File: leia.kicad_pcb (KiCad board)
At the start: 4 copper layers, 43 x 66 mm, 80 parts, among them P1 GND, P1000 ISO7816_NO, P3000 USB_FS_OTG, P513 TP1, P514 TP2, P515 TP3, P523 UART4, P542 TP4, P543 TP5, P545 TP7, P546 TP8, P547 TP9, P548 TP10, P572 DEBUG/PROG, P592 UART1, P595 I2C1_SCL, P596 I2C1_SDA, P6000 USB_FS_OTG, P828 XI, SW503 DFU, SW514 RESET, U1 LD1117S33TR, U300 USBLC6-2, U500 STM32F439VIT6, U600 USBLC6-2, U800 USB3300, Y2 ASEMB-24.000MHZ-LY-T

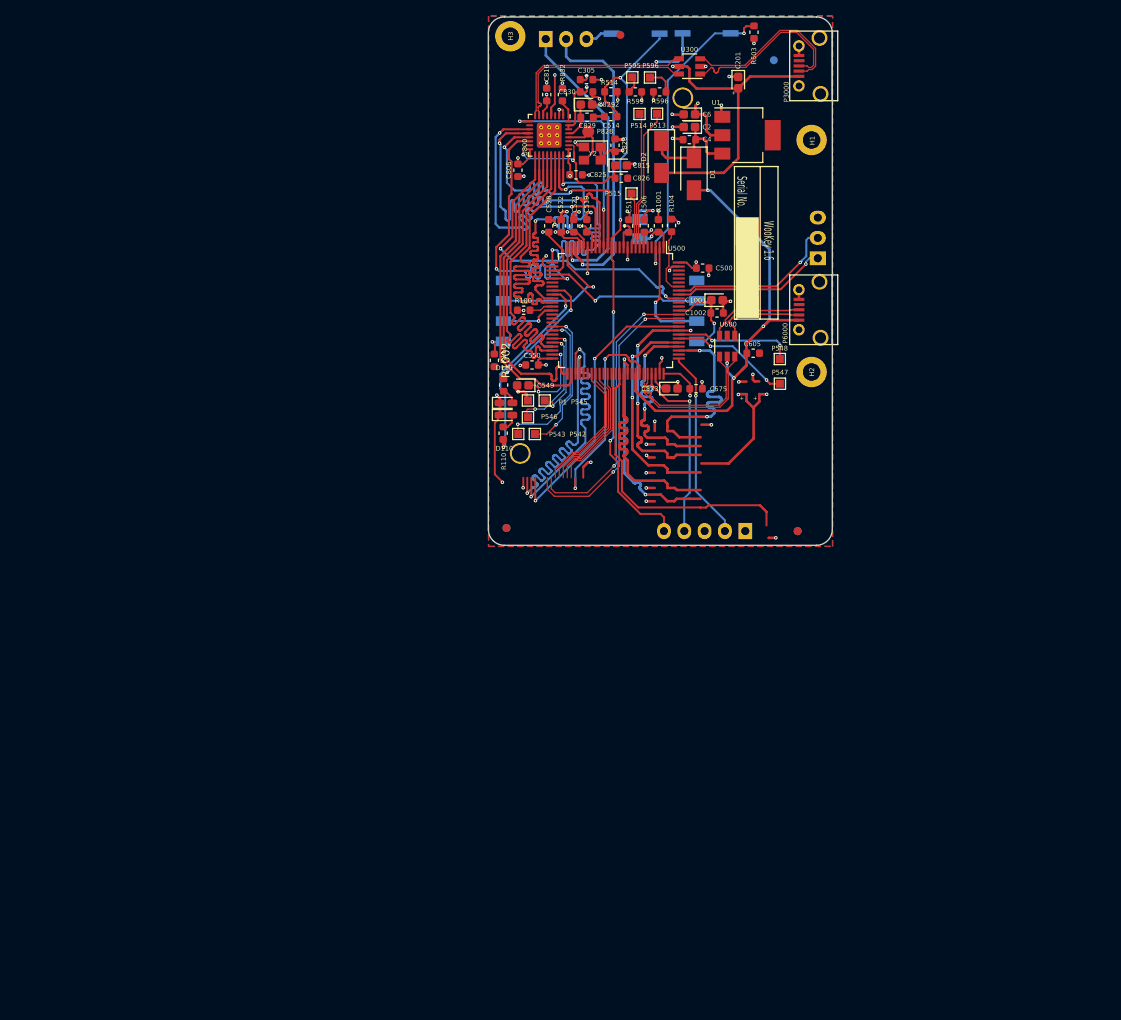
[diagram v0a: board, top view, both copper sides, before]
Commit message: [enhancement] add new file for chipwhisperer interface:iface_ufo.sch
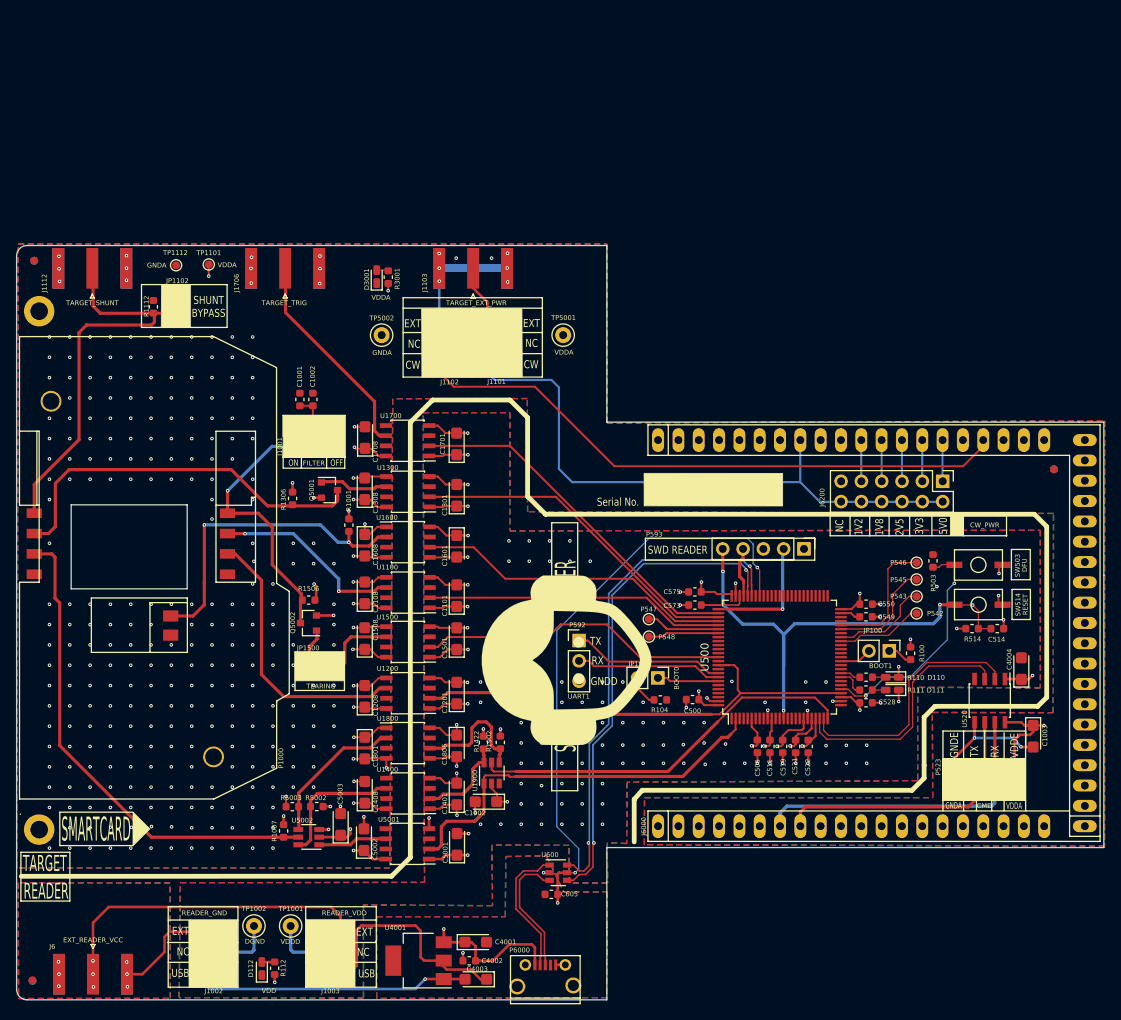
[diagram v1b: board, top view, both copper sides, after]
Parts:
- removed C2, C6: 10uF, Capacitor_Tantalum_SMD:CP_EIA-1608-08_AVX-J
- removed C201, C815, C8292: 4.7uF, Capacitor_Tantalum_SMD:CP_EIA-1608-08_AVX-J
- removed C305, C4, C806, C816, C825, C826, C829, C830: 100nF, Capacitor_SMD:C_0603_1608Metric
- removed C828: 0.01uF, Capacitor_SMD:C_0603_1608Metric
- removed D1, D2: STPS1L30A, Diode_SMD:D_SMA
- removed FID1, FID2, FID3: FIDUCIAL, Fiducials:Fiducial_1mm_Dia_2.54mm_Outer_CopperTop
- removed FID4, FID5, FID6: FIDUCIAL, Fiducials:Fiducial_1mm_Dia_2.54mm_Outer_CopperBottom
- removed H1: H1, Mounting_Holes:MountingHole_2.2mm_M2_ISO14580_Pad
- removed H2: H2, Mounting_Holes:MountingHole_2.2mm_M2_ISO14580_Pad
- removed H3: H3, Mounting_Holes:MountingHole_2.2mm_M2_ISO14580_Pad
- removed P1: GND, TestPoint:TestPoint_Pad_1.0x1.0mm
- removed P3000: USB_FS_OTG, leia:USB_Micro-B-MOLEX_105017-0001
- removed P513: TP1, TestPoint:TestPoint_Pad_1.0x1.0mm
- removed P514: TP2, TestPoint:TestPoint_Pad_1.0x1.0mm
- removed P515: TP3, TestPoint:TestPoint_Pad_1.0x1.0mm
- removed P572: DEBUG/PROG, Pin_Headers:Pin_Header_Straight_1x05
- removed P595: I2C1_SCL, TestPoint:TestPoint_Pad_1.0x1.0mm
- removed P596: I2C1_SDA, TestPoint:TestPoint_Pad_1.0x1.0mm
- removed P828: XI, Measurement_Points:Measurement_Point_Round-SMD-Pad_Small
- removed R1002: 10, Resistor_SMD:R_0603_1608Metric
- removed R595, R596: 47K, Resistor_SMD:R_0603_1608Metric
- removed R832: 12K [1%], Resistor_SMD:R_0603_1608Metric
- removed U1: LD1117S33TR, Package_TO_SOT_SMD:SOT-223
- removed U300: USBLC6-2, Package_TO_SOT_SMD:TSOT-23-6
- removed U800: USB3300, Package_DFN_QFN:QFN-32-1EP_5x5mm_P0.5mm_EP3.1x3.1mm_ThermalVias
- removed Y2: ASEMB-24.000MHZ-LY-T, Oscillator:Oscillator_SMD_Abracon_ASE-4Pin_3.2x2.5mm
- added C1003: 0.1uF 35V Tant, Capacitor_Tantalum_SMD:CP_EIA-3216-18_Kemet-A, F.Cu at (154.1, 129.7)
- added C1101: 0.1uF 35V Tant, Capacitor_Tantalum_SMD:CP_EIA-3216-18_Kemet-A, F.Cu at (82.0, 112.1)
- added C1108: 0.1uF 35V Tant, Capacitor_Tantalum_SMD:CP_EIA-3216-18_Kemet-A, F.Cu at (70.5, 111.8)
- added C1201: 0.1uF 35V Tant, Capacitor_Tantalum_SMD:CP_EIA-3216-18_Kemet-A, F.Cu at (82.0, 124.3)
- added C1208: 0.1uF 35V Tant, Capacitor_Tantalum_SMD:CP_EIA-3216-18_Kemet-A, F.Cu at (70.5, 124.7)
- added C1301: 0.1uF 35V Tant, Capacitor_Tantalum_SMD:CP_EIA-3216-18_Kemet-A, F.Cu at (82.0, 99.6)
- added C1308: 0.1uF 35V Tant, Capacitor_Tantalum_SMD:CP_EIA-3216-18_Kemet-A, F.Cu at (70.5, 98.8)
- added C1401: 0.1uF 35V Tant, Capacitor_Tantalum_SMD:CP_EIA-3216-18_Kemet-A, F.Cu at (82.0, 136.9)
- added C1408: 0.1uF 35V Tant, Capacitor_Tantalum_SMD:CP_EIA-3216-18_Kemet-A, F.Cu at (70.5, 136.7)
- added C1501: 0.1uF 35V Tant, Capacitor_Tantalum_SMD:CP_EIA-3216-18_Kemet-A, F.Cu at (82.0, 117.5)
- added C1508: 0.1uF 35V Tant, Capacitor_Tantalum_SMD:CP_EIA-3216-18_Kemet-A, F.Cu at (70.5, 117.5)
- added C1601: 0.1uF 35V Tant, Capacitor_Tantalum_SMD:CP_EIA-3216-18_Kemet-A, F.Cu at (82.0, 106.0)
- added C1608: 0.1uF 35V Tant, Capacitor_Tantalum_SMD:CP_EIA-3216-18_Kemet-A, F.Cu at (70.5, 105.8)
- added C1701: 0.1uF 35V Tant, Capacitor_Tantalum_SMD:CP_EIA-3216-18_Kemet-A, F.Cu at (82.0, 93.2)
- added C1708: 0.1uF 35V Tant, Capacitor_Tantalum_SMD:CP_EIA-3216-18_Kemet-A, F.Cu at (70.6, 92.4)
- added C1801: 0.1uF 35V Tant, Capacitor_Tantalum_SMD:CP_EIA-3216-18_Kemet-A, F.Cu at (70.5, 131.2)
- added C1806: 0.1uF 35V Tant, Capacitor_Tantalum_SMD:CP_EIA-3216-18_Kemet-A, F.Cu at (82.0, 130.9)
- added C1902: 0.1uF 35V Tant, Capacitor_Tantalum_SMD:CP_EIA-3216-18_Kemet-A, F.Cu at (85.7, 137.9)
- added C4001: 10uF, Capacitor_Tantalum_SMD:CP_EIA-3216-18_Kemet-A, F.Cu at (84.4, 155.4)
- added C4002: 100nF, Capacitor_SMD:C_0603_1608Metric, F.Cu at (83.6, 157.8)
- added C4003: 10uF, Capacitor_Tantalum_SMD:CP_EIA-3216-18_Kemet-A, F.Cu at (84.4, 160.1)
- added C4004: 0.1uF 35V Tant, Capacitor_Tantalum_SMD:CP_EIA-3216-18_Kemet-A, F.Cu at (152.6, 121.3)
- added C5001: 0.1uF 35V Tant, Capacitor_Tantalum_SMD:CP_EIA-3216-18_Kemet-A, F.Cu at (82.1, 143.2)
- added C5002: 0.1uF 35V Tant, Capacitor_Tantalum_SMD:CP_EIA-3216-18_Kemet-A, F.Cu at (70.4, 142.6)
- added C5003: 0.1uF 35V Tant, Capacitor_Tantalum_SMD:CP_EIA-3216-18_Kemet-A, F.Cu at (67.5, 140.7)
- added D112: VDD, LED_SMD:LED_0603_1608Metric_Castellated, F.Cu at (57.7, 158.8)
- added D3001: VDDA, LED_SMD:LED_0603_1608Metric_Castellated, F.Cu at (72.0, 72.3)
- added FID1001: FIDUCIAL-RESCUE-rescue, Fiducial:Fiducial_1mm_Mask2mm, B.Cu at (29.0, 160.3)
- added FID1002: FIDUCIAL-RESCUE-rescue, Fiducial:Fiducial_1mm_Mask2mm, F.Cu at (29.2, 70.3)
- added FID1003: FIDUCIAL-RESCUE-rescue, Fiducial:Fiducial_1mm_Mask2mm, B.Cu at (29.2, 70.3)
- added FID1004: FIDUCIAL-RESCUE-rescue, Fiducial:Fiducial_1mm_Mask2mm, F.Cu at (156.7, 96.3)
- added FID1005: FIDUCIAL-RESCUE-rescue, Fiducial:Fiducial_1mm_Mask2mm, B.Cu at (156.7, 96.3)
- added FID1006: FIDUCIAL-RESCUE-rescue, Fiducial:Fiducial_1mm_Mask2mm, F.Cu at (29.0, 160.2)
- added G***: LOGO, leia:Leia-medium, F.Cu at (95.8, 120.2)
- added HOLE1: HOLE, MountingHole:MountingHole_2.2mm_M2_ISO14580_Pad, F.Cu at (29.8, 141.4)
- added HOLE2: HOLE, MountingHole:MountingHole_2.2mm_M2_ISO14580_Pad, F.Cu at (29.8, 76.6)
- added J1001: FILTER, Connector_PinHeader_2.54mm:PinHeader_2x03_P2.54mm_Vertical, F.Cu at (61.7, 93.5)
- added J1002: READER_GND, Connector_PinHeader_2.54mm:PinHeader_2x03_P2.54mm_Vertical, F.Cu at (52.9, 159.2)
- added J1003: READER_VDD, Connector_PinHeader_2.54mm:PinHeader_2x03_P2.54mm_Vertical, F.Cu at (67.5, 159.2)
- added J1101: TARGET_PWR, Connector_PinHeader_2.54mm:PinHeader_2x03_P2.54mm_Vertical, F.Cu at (88.4, 83.1)
- added J1102: TARGET_GND, Connector_PinHeader_2.54mm:PinHeader_2x03_P2.54mm_Vertical, F.Cu at (82.0, 83.1)
- added J1103: TARGET_EXT_PWR, Connector_Coaxial:SMA_Amphenol_132289_EdgeMount, F.Cu at (84.1, 71.2)
- added J1112: TARGET_SHUNT, Connector_Coaxial:SMA_Amphenol_132289_EdgeMount, F.Cu at (36.5, 71.2)
- added J1706: TARGET_TRIG, Connector_Coaxial:SMA_Amphenol_132289_EdgeMount, F.Cu at (60.6, 71.2)
- added J6: EXT_READER_VCC, Connector_Coaxial:SMA_Amphenol_132289_EdgeMount, F.Cu at (36.6, 159.5)
- added J6000: CW308_TARGETCON, leia:CW308T_CONNBOARD, F.Cu at (107.2, 141.0)
- added J6200: CW_PWR, Connector_PinHeader_2.54mm:PinHeader_2x06_P2.54mm_Vertical, F.Cu at (142.8, 97.8)
- added JP100: BOOT1, Connector_PinHeader_2.54mm:PinHeader_1x02_P2.54mm_Vertical, F.Cu at (136.1, 119.0)
- added JP101: BOOT0, Connector_PinHeader_2.54mm:PinHeader_1x02_P2.54mm_Vertical, F.Cu at (107.2, 122.4)
- added JP1102: SHUNT Bypass, Connector_PinHeader_2.54mm:PinHeader_1x02_P2.54mm_Vertical, F.Cu at (46.9, 77.2)
- added JP1500: TEARING, Connector_PinHeader_2.54mm:PinHeader_1x02_P2.54mm_Vertical, F.Cu at (66.2, 121.0)
- added P593: SWD, Connector_PinHeader_2.54mm:PinHeader_1x05_P2.54mm_Vertical, F.Cu at (125.4, 106.3)
- added Q5001: BSS84, Package_TO_SOT_SMD:SOT-23, F.Cu at (66.1, 98.9)
- added Q5002: BSS84, Package_TO_SOT_SMD:SOT-23, F.Cu at (63.5, 115.6)
- added R1007: 22k, Resistor_SMD:R_0603_1608Metric, F.Cu at (60.4, 141.6)
- added R1112: 0.1 1%, Resistor_SMD:R_0603_1608Metric, F.Cu at (44.1, 76.0)
- added R112: 470, Resistor_SMD:R_0603_1608Metric, F.Cu at (59.3, 158.7)
- added R1306: 10k, Resistor_SMD:R_0603_1608Metric, F.Cu at (61.5, 100.0)
- added R1422: 22k, Resistor_SMD:R_0603_1608Metric, F.Cu at (85.4, 130.5)
- added R1506: 10k, Resistor_SMD:R_0603_1608Metric, F.Cu at (63.5, 112.7)
- added R1902: 22k, Resistor_SMD:R_0603_1608Metric, F.Cu at (87.5, 130.5)
- added R3001: 470, Resistor_SMD:R_0603_1608Metric, F.Cu at (73.5, 72.3)
- added R5002: DNP, Resistor_SMD:R_0603_1608Metric, F.Cu at (64.5, 138.5)
- added R5003: DNP, Resistor_SMD:R_0603_1608Metric, F.Cu at (61.5, 138.5)
- added TP1001: VDDD, TestPoint_Keystone_5000-5004_Miniature, F.Cu at (61.3, 153.4)
- added TP1002: DGND, TestPoint_Keystone_5000-5004_Miniature, F.Cu at (56.7, 153.4)
- added TP1101: VDDA, TestPoint:TestPoint_Pad_D1.0mm, F.Cu at (51.0, 70.7)
- added TP1112: GNDA, TestPoint:TestPoint_Pad_D1.0mm, F.Cu at (46.9, 70.8)
- added TP5001: VDDA, TestPoint_Keystone_5000-5004_Miniature, F.Cu at (95.3, 79.6)
- added TP5002: GNDA, TestPoint_Keystone_5000-5004_Miniature, F.Cu at (72.6, 79.6)
- added U1100: FOD8001, Package_SO:SOIC-8_3.9x4.9mm_P1.27mm, F.Cu at (75.9, 111.8)
- added U1200: FOD8001, Package_SO:SOIC-8_3.9x4.9mm_P1.27mm, F.Cu at (75.9, 124.3)
- added U1300: FOD8001, Package_SO:SOIC-8_3.9x4.9mm_P1.27mm, F.Cu at (75.9, 99.2)
- added U1400: FOD8001, Package_SO:SOIC-8_3.9x4.9mm_P1.27mm, F.Cu at (75.9, 136.9)
- added U1500: FOD8001, Package_SO:SOIC-8_3.9x4.9mm_P1.27mm, F.Cu at (75.9, 117.9)
- added U1600: FOD8001, Package_SO:SOIC-8_3.9x4.9mm_P1.27mm, F.Cu at (75.9, 105.5)
- added U1700: FOD8001, Package_SO:SOIC-8_3.9x4.9mm_P1.27mm, F.Cu at (75.9, 92.8)
- added U1800: FOD8001, Package_SO:SOIC-8_3.9x4.9mm_P1.27mm, F.Cu at (75.9, 130.6)
- added U1900: ADG719-EP, Package_TO_SOT_SMD:TSOT-23-6, F.Cu at (86.4, 134.3)
- added U4001: LD1117S33TR, Package_TO_SOT_SMD:SOT-223, F.Cu at (77.3, 157.8)
- added U5001: FOD8001, Package_SO:SOIC-8_3.9x4.9mm_P1.27mm, F.Cu at (75.9, 143.2)
- added U5002: ADG719-EP, Package_TO_SOT_SMD:TSOT-23-6, F.Cu at (63.5, 142.3)
- added U520: FOD8012A, Package_SO:SOIC-8_3.9x4.9mm_P1.27mm, F.Cu at (148.7, 125.3)
- C1001, C549, C573: footprint Capacitor_Tantalum_SMD:CP_EIA-1608-08_AVX-J -> Capacitor_SMD:C_0603_1608Metric
- P1000, SW503, SW514: moved to F.Cu
- P523: value UART4 -> CMD; footprint Pin_Headers:Pin_Header_Straight_1x03 -> Connector_PinHeader_2.54mm:PinHeader_2x04_P2.54mm_Vertical; moved to F.Cu
- P542, P543, P545, P546, P547, P548: footprint TestPoint:TestPoint_Pad_1.0x1.0mm -> TestPoint:TestPoint_Pad_D1.0mm
- P592: footprint Pin_Headers:Pin_Header_Straight_1x03 -> Connector_PinHeader_2.54mm:PinHeader_1x03_P2.54mm_Vertical; moved to F.Cu
- P6000: value USB_FS_OTG -> USB_FS
- R1001: value 10K -> 20k
- U500: footprint Housings_QFP:LQFP-100_14x14mm_Pitch0.5mm -> Package_QFP:TQFP-100_14x14mm_P0.5mm
- U600: footprint Package_TO_SOT_SMD:TSOT-23-6 -> Package_TO_SOT_SMD:SOT-23-6
- moved P523 108.5 mm to (151.8, 133.8)
- moved P1000 101.2 mm to (51.6, 132.3), turned to 270 degrees
- moved P6000 91.3 mm to (93.1, 161.0), turned to 0 degrees
- moved SW514 83.3 mm to (147.2, 113.3)
- moved R514 80.9 mm to (146.4, 116.3), turned to 0 degrees
- moved C514 80.2 mm to (149.6, 116.3), turned to 0 degrees
- moved SW503 74.6 mm to (147.2, 108.3)
- moved C605 72.2 mm to (93.9, 149.5), turned to 180 degrees
- moved C522 72.0 mm to (126.0, 131.0), turned to 270 degrees
- moved C528 71.6 mm to (133.2, 125.5), turned to 0 degrees
- moved C521 70.7 mm to (124.4, 131.0), turned to 270 degrees
- moved R503 69.8 mm to (141.6, 107.8), turned to 90 degrees
- moved C519 69.5 mm to (122.8, 131.0), turned to 270 degrees
- moved U600 69.1 mm to (94.7, 146.8), turned to 0 degrees
- moved C511 67.4 mm to (121.2, 131.0), turned to 270 degrees
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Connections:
- net LED0 renamed /cpu/LED0_PC4
- net LED1 renamed /cpu/LED1_PC5
- C1001 pad 1: /cpu/CARD_POWER -> Net-(C1001-Pad1)
- C1001 pad 2: GND -> GNDA
- C1002 pad 1: /cpu/CARD_POWER -> Net-(C1001-Pad1)
- C1002 pad 2: GND -> GNDA
- C500 pad 1: +3V3 -> VDD
- C500 pad 2: GND -> GNDD
- C506 pad 1: +3V3 -> VDD
- C506 pad 2: GND -> GNDD
- C511 pad 1: +3V3 -> VDD
- C511 pad 2: GND -> GNDD
- C514 pad 2: GND -> GNDD
- C519 pad 1: +3V3 -> VDD
- C519 pad 2: GND -> GNDD
- C521 pad 1: +3V3 -> VDD
- C521 pad 2: GND -> GNDD
- C522 pad 1: +3V3 -> VDD
- C522 pad 2: GND -> GNDD
- C528 pad 1: +3V3 -> VDD
- C528 pad 2: GND -> GNDD
- C549 pad 2: GND -> GNDD
- C550 pad 1: +3V3 -> VDD
- C550 pad 2: GND -> GNDD
- C573 pad 2: GND -> GNDD
- C575 pad 1: +3V3 -> VDD
- C575 pad 2: GND -> GNDD
- C605 pad 2: GND -> GNDPWR
- D110 pad 1: GND -> GNDD
- D111 pad 1: GND -> GNDD
- P1000 pad C1: /cpu/CARD_POWER -> /dfu smartcard/CRD_PWR
- P1000 pad C2: /cpu/CARD_RESET -> /dfu smartcard/CRD_RST
- P1000 pad C3: /cpu/CARD_CLK -> /dfu smartcard/CRD_CLK
- P1000 pad C5: Net-(P1000-PadC5) -> /GNDCARD
- P1000 pad C6: /cpu/CARD_VPP -> /dfu smartcard/CRD_VPP
- P1000 pad C7: /cpu/CARD_IO -> /dfu smartcard/CRD_IO
- P1000 pad SW1: /cpu/CARD_CT -> /dfu smartcard/CRD_CT
- P1000 pad SW2: GND -> GNDA
- P523 pad 1: /cpu/UART4_RX_PA1 -> /VDD_CONSOLE
- P523 pad 2: /cpu/UART4_TX_PA0 -> VDDA
- P523 pad 3: GND -> /RX_CONSOLE
- P592 pad 3: GND -> GNDD
- P6000 pad 5: GND -> GNDPWR
- P6000 pad 6: GND -> GNDPWR
- R100 pad 1: +3V3 -> VDD
- R100 pad 2: /cpu/BOOT1 -> Net-(JP100-Pad1)
- R1001 pad 1: +3V3 -> VDDA
- R1001 pad 2: /cpu/CARD_CT -> /dfu smartcard/CRD_CT
- R104 pad 1: /cpu/BOOT0 -> Net-(JP101-Pad2)
- R104 pad 2: GND -> GNDD
- R503 pad 2: GND -> GNDD
- R514 pad 1: +3V3 -> VDD
- SW503 pad 1: +3V3 -> VDD
- SW514 pad 2: GND -> GNDD
- U500 pad 1: /cpu/CARD_CT -> (no net)
- U500 pad 10: GND -> GNDD
- U500 pad 100: +3V3 -> VDD
- U500 pad 11: +3V3 -> VDD
- U500 pad 15: /cpu/USB_HS_ULPI_STP -> (no net)
- U500 pad 16: /cpu/USB_HS_HARD_RESET -> (no net)
- U500 pad 17: /cpu/USB_HS_ULPI_DIR -> (no net)
- U500 pad 18: /cpu/USB_HS_ULPI_NXT -> (no net)
- U500 pad 19: +3V3 -> VDD
- U500 pad 2: /cpu/CARD_RESET -> /cpu/CARD_~R~W
- U500 pad 20: GND -> GNDD
- U500 pad 21: +3V3 -> VDD
- U500 pad 22: +3V3 -> VDD
- U500 pad 23: /cpu/UART4_TX_PA0 -> /TX_CMD
- U500 pad 24: /cpu/UART4_RX_PA1 -> /RX_CMD
- U500 pad 26: /cpu/USB_HS_ULPI_D0 -> (no net)
- U500 pad 27: GND -> GNDD
- U500 pad 28: +3V3 -> VDD
- U500 pad 3: /cpu/DFU -> (no net)
- U500 pad 30: /cpu/USB_HS_ULPI_CLK -> /cpu/DFU
- U500 pad 35: /cpu/USB_HS_ULPI_D1 -> (no net)
- U500 pad 36: /cpu/USB_HS_ULPI_D2 -> (no net)
- U500 pad 38: /cpu/CARD_VPP -> (no net)
- U500 pad 47: /cpu/USB_HS_ULPI_D3 -> (no net)
- U500 pad 48: /cpu/USB_HS_ULPI_D4 -> (no net)
- U500 pad 50: +3V3 -> VDD
- U500 pad 51: /cpu/USB_HS_ULPI_D5 -> (no net)
- U500 pad 52: /cpu/USB_HS_ULPI_D6 -> (no net)
- U500 pad 6: +3V3 -> VDD
- U500 pad 7: /cpu/TP1 -> (no net)
- U500 pad 72: /cpu/TMS/SWIO -> /cpu/TMS
- U500 pad 74: GND -> GNDD
- U500 pad 75: +3V3 -> VDD
- U500 pad 76: /cpu/TCK/SWCLK -> /cpu/TCK
- U500 pad 77: (no net) -> /cpu/TRIGGER
- U500 pad 78: (no net) -> /cpu/CARD_VPP
- U500 pad 79: (no net) -> /cpu/CARD_CT
- U500 pad 8: /cpu/TP2 -> (no net)
- U500 pad 80: (no net) -> /cpu/CARD_RESET
- U500 pad 88: /cpu/CARD_POWER -> /cpu/CARD_PWR_EN
- U500 pad 9: /cpu/TP3 -> (no net)
- U500 pad 90: (no net) -> /cpu/CARD_CLK
- U500 pad 91: /cpu/USB_HS_ULPI_D7 -> (no net)
- U500 pad 99: GND -> GNDD
- U600 pad 2: GND -> GNDPWR
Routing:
- net (no net): track 493.1 -> 0.00 mm, vias 23 -> 0
- net VDD: track 0.00 -> 110.0 mm, vias 0 -> 26
- net +3V3: track 108.5 -> 0.00 mm, vias 31 -> 0
- net GNDD: track 0.00 -> 80.4 mm, vias 0 -> 118
- net VCOM: track 0.00 -> 78.1 mm
- net VDDA: track 0.00 -> 61.4 mm, vias 0 -> 18
- net /dfu smartcard/CRD_IO: track 0.00 -> 61.1 mm
- net /cpu/CARD_~R~W: track 0.00 -> 53.7 mm
- net /GNDCARD: track 0.00 -> 51.7 mm
- net /dfu smartcard/CRD_VPP: track 0.00 -> 47.9 mm
- net /cpu/USB_HS_ULPI_D1: track 46.8 -> 0.00 mm, vias 2 -> 0
- net /cpu/USB_HS_VBUS: track 45.8 -> 0.00 mm, vias 3 -> 0
- net /cpu/TRIGGER: track 0.00 -> 44.6 mm
- net /cpu/USB_HS_ULPI_DIR: track 44.3 -> 0.00 mm, vias 2 -> 0
- net /cpu/USB_FS_D-: track 19.9 -> 61.7 mm, vias 0 -> 2
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- added copper zone on B.Cu, net /EXT_READER_GND
- added copper zone on F.Cu, net /EXT_READER_GND
- added copper zone on In1.Cu, net /EXT_READER_GND
- added copper zone on In2.Cu, net /EXT_READER_VCC
- added copper zone on In2.Cu, net /cpu/USB_FS_VBUS
- added copper zone on B.Cu, net GNDA
- added copper zone on F.Cu, net GNDA
- added copper zone on In1.Cu, net GNDA
- added copper zone on B.Cu, net GNDD
- added copper zone on F.Cu, net GNDD
- added copper zone on In1.Cu, net GNDD
- added copper zone on B.Cu, net GNDPWR
- added copper zone on F.Cu, net GNDPWR
- added copper zone on In1.Cu, net GNDPWR
- added copper zone on In2.Cu, net VDD
- added copper zone on In2.Cu, net VDDA
- removed copper zone on In2Power.Cu, net +3V3
- removed copper zone on In2Power.Cu, net /cpu/USB_FS_VBUS
- removed copper zone on In2Power.Cu, net /cpu/USB_HS_VBUS
- removed copper zone on B.Cu, net GND
- removed copper zone on F.Cu, net GND
- removed copper zone on In1GroundPlan.Cu, net GND
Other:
- board size 43 x 66 mm -> 135.9 x 94.3 mm
- net class Default: clearance 0.127 -> 0.2; via_dia 0.44 -> 0.8; via_drill 0.2 -> 0.4
- net class Power: clearance 0.127 -> 0.15; trace_width 0.127 -> 0.25
- rule trace_clearance: 0.127 -> 0.2
- rule via_min_size: 0.44 -> 0.2
- board text added: "1"
- board text added: "10"
- board text added: "11"
- board text added: "12"
- board text added: "13"
- board text added: "14"
- board text added: "15"
- board text added: "16"
- board text added: "17"
- board text added: "18"
- board text added: "19"
- board text added: "1V2"
- board text added: "1V8"
- board text added: "2"
- board text added: "20"
- board text added: "21"
- board text added: "22"
- board text added: "23"
- board text added: "24"
- board text added: "25"
- board text added: "26"
- board text added: "27"
- board text added: "28"
- board text added: "29"
- board text added: "2V5"
- board text added: "3"
- board text added: "30"
- board text added: "31/32"
- board text added: "33/34"
- board text added: "35/36"
- board text added: "37/38"
- board text added: "39/40"
- board text added: "3V3"
- board text added: "4"
- board text added: "5"
- board text added: "5V0"
- board text added: "6"
- board text added: "7"
- board text added: "8"
- board text added: "9"
- board text added: "CW"
- board text added: "EXT"
- board text added: "GNDA"
- board text added: "GNDD"
- board text added: "GNDE"
- board text added: "NC"
- board text added: "OFF"
- board text added: "ON"
- board text added: "READER"
- board text added: "RX"
- board text added: "SHUNT BYPASS"
- board text added: "SMART READER"
- board text added: "SMARTCARD"
- board text added: "SWD READER"
- board text added: "TARGET"
- board text added: "TX"
- board text added: "The board is a 4 Layer Stackup is as follows: ============================================ Solder resist: 20 µm Cu - L1 (TOP): 35 µm PP - 1 : 175 µm (7628LR) e = 4.2 Cu - L2 : 17.5 µm Core - 1 : 1150 µm e = 4.3 Cu - L3 : 17.5 µm PP - 2 : 175 µm (7628LR) e = 4.2 Cu - L4 (BOT): 35 µm Solder resist: 20 µm 1645 µm Tolerance +/-10% (min 1480.5 µm .. max 1809.5 µm) Substrate is: VENTEC: FR4 - VT481 - T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"
- board text added: "The board is a 4 Layer Stackup is as follows: ============================================ Solder resist: 20 µm Cu - L1 (TOP): 35 µm PP - 1 : 175 µm Cu - L2 : 17.5 µm Core - 1 : 1150 µm Cu - L3 : 17.5 µm PP - 2 : 175 µm Cu - L4 (BOT): 35 µm Solder resist: 20 µm 1645 µm Tolerance +/-10% (min 1480.5 µm .. max 1809.5 µm)"
- board text added: "USB"
- board text added: "VDDA"
- board text added: "VDDE"
- board text removed: "DFU"
- board text removed: "RESET"
- board text removed: "The current 4 layer 1.6mm board stackup is as follows: Thickness Layer ======================================== Outer layers 1 oz base copper foil Inner layers 0.5 oz base copper foil Electroless Nickel Immersion Gold (ENIG) surface finish solder resist 0.0254mm copper 0.0356mm L1 (TOP) FR408 prepreg 0.1702mm copper 0.0178mm L2 (GND) FR408 1.1938mm copper 0.0178mm L3 (PWR) FR408 prepreg 0.1702mm 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"
- board text removed: "WooKey 1.6"
